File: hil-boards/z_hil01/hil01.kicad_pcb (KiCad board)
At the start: 2 copper layers, 61.7 x 30.5 mm, 40 parts, among them J1 USB_C_Receptacle_USB2.0, J2 Conn_01x03_Male, U1 ADUM4160, U2 MAX485E, U3 CH340G, Y1 Crystal

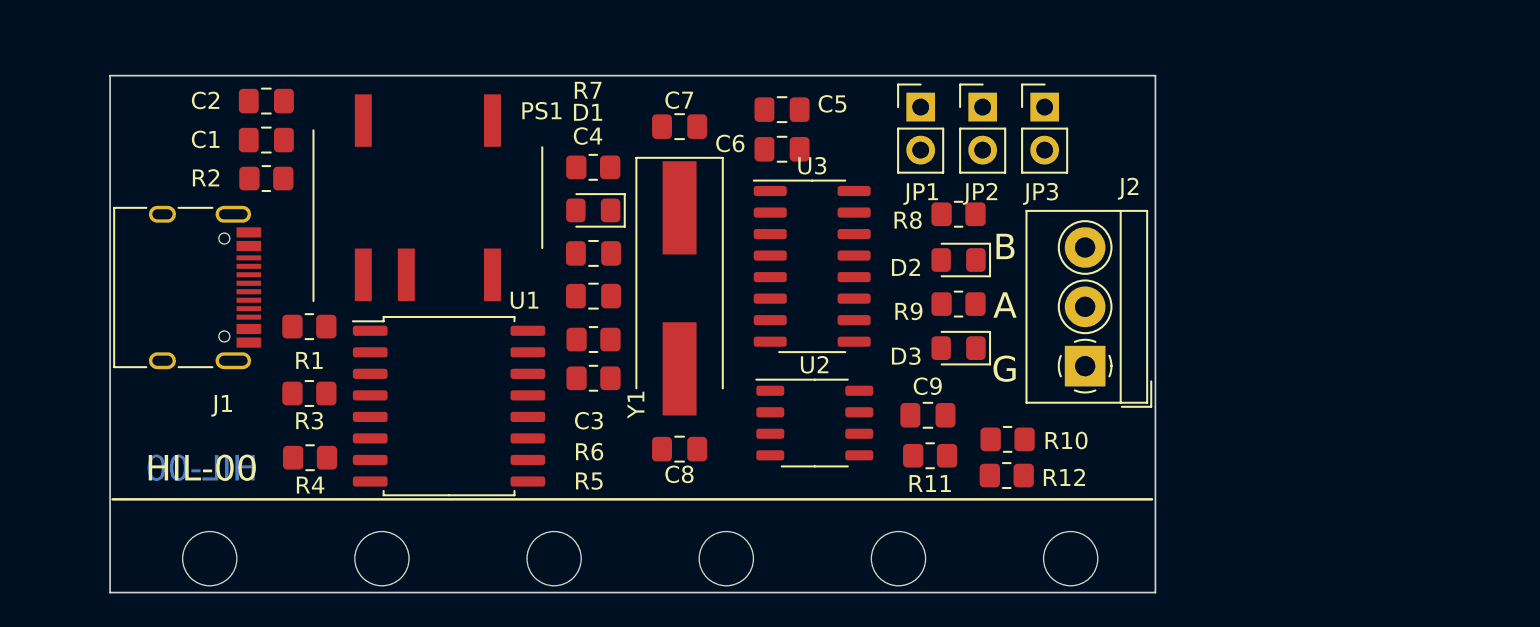
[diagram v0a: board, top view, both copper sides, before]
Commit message: all elements placed
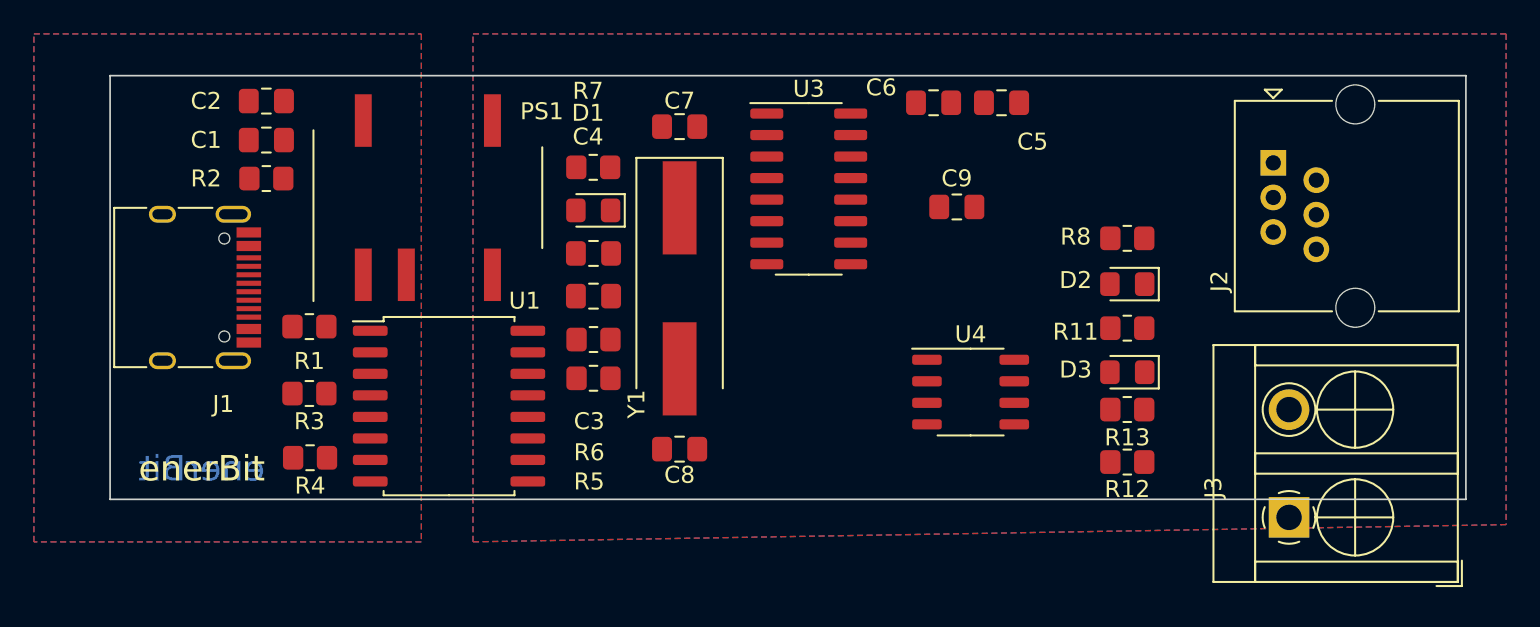
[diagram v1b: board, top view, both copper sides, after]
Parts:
- removed JP1, JP2, JP3: Jumper_2_Open, Connector_PinHeader_2.54mm:PinHeader_1x02_P2.54mm_Vertical
- removed R10: 560, Resistor_SMD:R_0805_2012Metric_Pad1.20x1.40mm_HandSolder
- removed the R11 at (148.4, 122.4)
- removed REF**2, REF**3, REF**4, REF**5, REF**6, REF**7: MountingHole_3.2mm_M3, MountingHole:MountingHole_3.2mm_M3
- removed U2: MAX485E, Package_SO:SOP-8_3.9x4.9mm_P1.27mm
- added J3: Conn_01x02_Female, Connector_Kefa:TerminalBlock_Kefa_1x02_P6.35mm_Horizontal, F.Cu at (169.6, 126.1)
- added R13: 100, Resistor_SMD:R_0805_2012Metric_Pad1.20x1.40mm_HandSolder, F.Cu at (160.0, 119.7)
- added U4: MAX485E, Package_SO:SO-8_3.9x4.9mm_P1.27mm, F.Cu at (150.8, 118.7)
- J2: value Conn_01x03_Male -> RJ25; footprint TerminalBlock_4Ucon:TerminalBlock_4Ucon_1x03_P3.50mm_Horizontal -> Connector_RJ:RJ25_Wayconn_MJEA-660X1_Horizontal
- R12: value 560 -> 100
- moved J2 16.3 mm to (168.6, 105.1)
- moved C5 13.0 mm to (152.6, 101.6)
- moved C9 12.4 mm to (150.0, 107.7)
- moved R11 10.1 mm to (160.0, 114.9)
- moved D2 10.1 mm to (160.0, 112.3)
- moved D3 10.1 mm to (160.0, 117.5)
- moved R8 10.1 mm to (160.0, 109.6)
- moved C6 9.35 mm to (148.6, 101.6)
- moved R12 7.16 mm to (160.0, 122.8)
- moved U3 4.58 mm to (141.2, 106.7)
- renumbered R9 to R11
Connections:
- net +5V renamed VCC
- J2 pad 1: GND2 -> unconnected-(J2-Pad1)
- J2 pad 2: /RS485_A -> unconnected-(J2-Pad2)
- J2 pad 3: /RS485_B -> unconnected-(J2-Pad3)
- R12 pad 1: GND2 -> Net-(R12-Pad1)
- R12 pad 2: Net-(JP3-Pad2) -> GND2
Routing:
- added copper zone on B.Cu, net GND1
- added copper zone on F.Cu, net GND1
- added copper zone on B.Cu, net GND2
- added copper zone on F.Cu, net GND2
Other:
- board size 61.7 x 30.5 mm -> 80 x 25 mm
- board text added: "3.3V"
- board text added: "5V"
- board text added: "AUTO"
- board text added: "CTS"
- board text added: "DTR"
- board text added: "EN"
- board text added: "GND"
- board text added: "IO0"
- board text added: "MANUAL"
- board text added: "RJ1"
- board text added: "RJ2"
- board text added: "RJ3"
- board text added: "RJ4"
- board text added: "RJ5"
- board text added: "RTS"
- board text added: "RX"
- board text added: "TX"
- board text added: "VIO"
- board text added: "enerBit"
- board text removed: "A"
- board text removed: "B"
- board text removed: "DISABLE"
- board text removed: "ENABLE"
- board text removed: "G"
- board text removed: "HIL-00"
- board text removed: "JP1"
- board text removed: "JP2"
- board text removed: "JP3"
- board text removed: "PLL-DW"
- board text removed: "PLL-UP"
- board text removed: "TERM"
